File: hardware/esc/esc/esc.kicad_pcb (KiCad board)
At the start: 4 copper layers, 120 x 80 mm, 291 parts, among them IC1 IR2136SPBF, IC2 IR2136SPBF, IC3 IR2136SPBF, IC4 IR2136SPBF, IC5 IR2136SPBF, IC6 IR2136SPBF, IC7 TLA2528IRTER, IC8 MP9486AGN-Z, J1 USB-C, J10 GPIO, J11 Conn_01x08_Pin, J2 DEBUG, J3 TEMP-GPIO, Q1 NMOS, Q10 NMOS, Q11 NMOS, Q12 NMOS, Q13 NMOS, Q14 NMOS, Q15 NMOS, Q16 NMOS, Q17 NMOS, Q18 NMOS, Q19 NMOS, Q2 NMOS, Q20 NMOS, Q21 NMOS, Q22 NMOS, Q23 NMOS, Q24 NMOS, Q25 NMOS, Q26 NMOS, Q27 NMOS, Q28 NMOS, Q29 NMOS, Q3 NMOS, Q30 NMOS, Q31 NMOS, Q32 NMOS, Q33 NMOS, Q34 NMOS, Q35 NMOS, Q36 NMOS, Q37 SMALL, Q38 SMALL, Q4 NMOS, Q5 NMOS, Q6 NMOS, Q7 NMOS, Q8 NMOS, Q9 NMOS, SW1 SW_Push, SW2 SW_Push, U1 RP2354B, U10 INA240A2PW, U11 INA240A2PW, U12 INA240A2PW, U14 TMP110D, U15 TMP110D, U16 AZ1117CH2-3.3, U2 INA240A2PW, U3 INA240A2PW, U4 INA240A2PW, U5 INA240A2PW, U6 INA240A2PW, U8 INA240A2PW, U9 INA240A2PW, Y1 12MHz

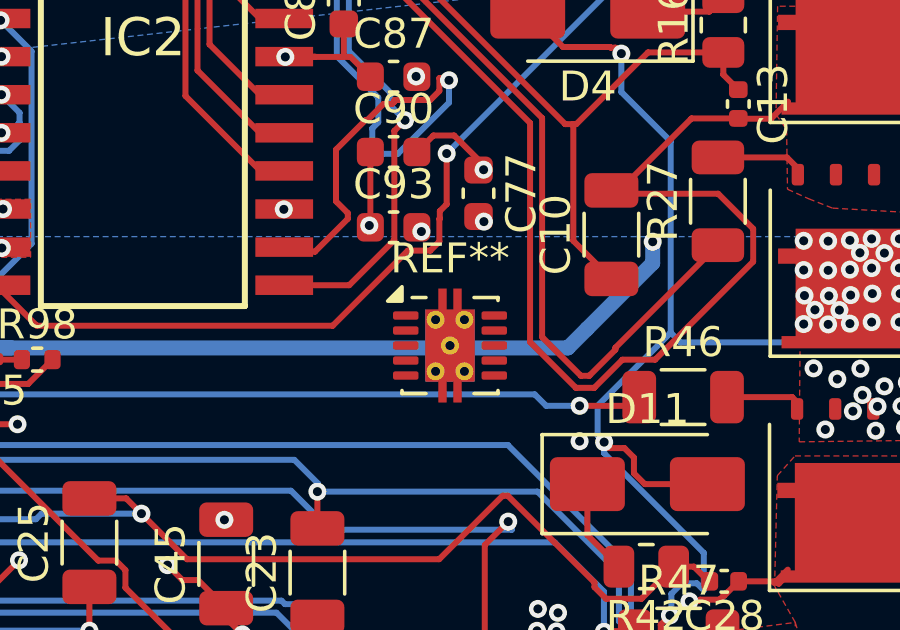
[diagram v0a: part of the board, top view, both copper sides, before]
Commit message: Auto-sync ESC PCB 2026-05-11 02:34:28
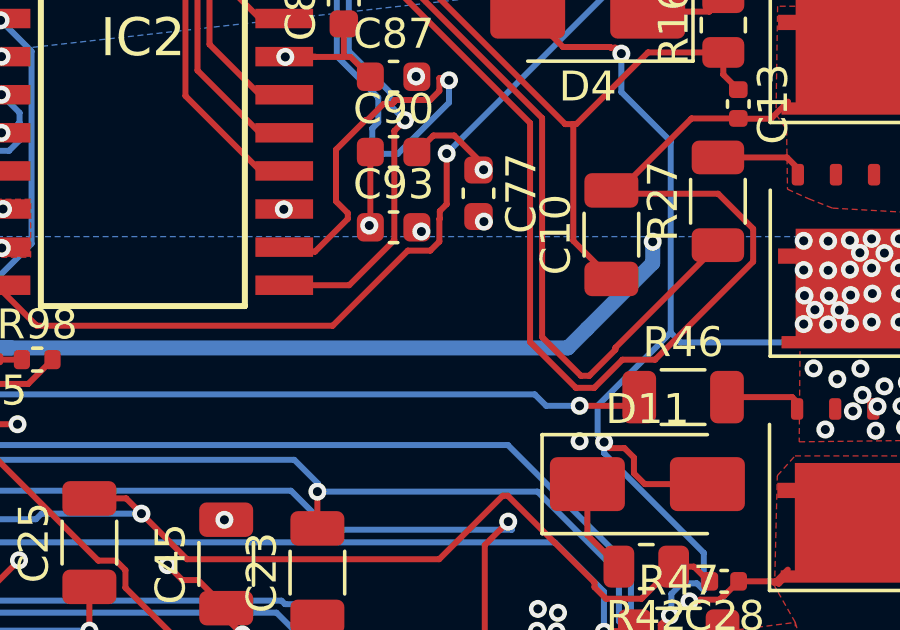
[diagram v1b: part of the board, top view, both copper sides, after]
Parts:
- removed REF**: VSON-10-1EP_3x3mm_P0.5mm_EP1.65x2.4mm_ThermalVias, Package_SON:VSON-10-1EP_3x3mm_P0.5mm_EP1.65x2.4mm_ThermalVias

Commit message: Auto-sync ESC PCB 2026-05-11 00:51:51
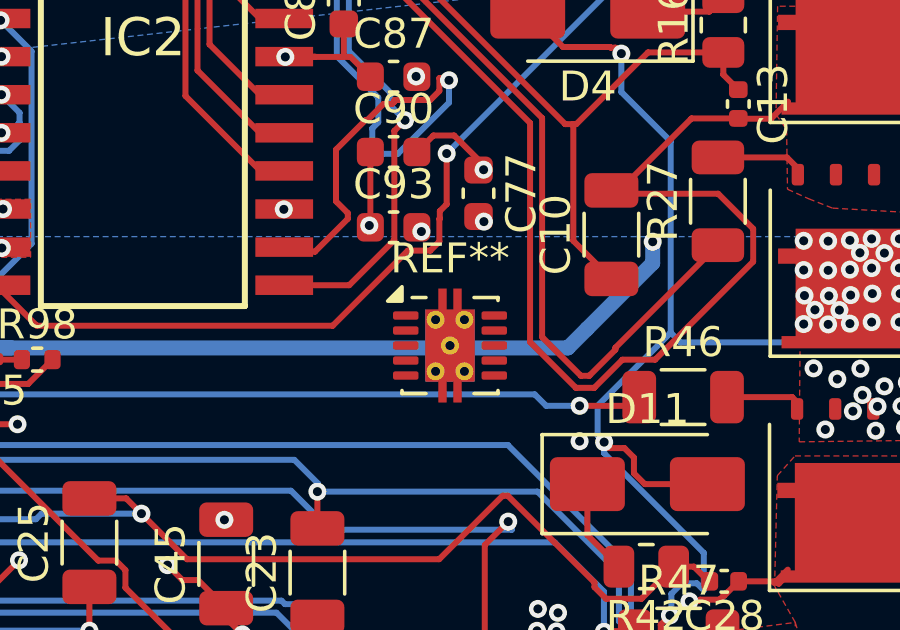
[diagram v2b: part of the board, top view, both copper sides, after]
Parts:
- added REF**: VSON-10-1EP_3x3mm_P0.5mm_EP1.65x2.4mm_ThermalVias, Package_SON:VSON-10-1EP_3x3mm_P0.5mm_EP1.65x2.4mm_ThermalVias, F.Cu at (98.4, 45.6)
